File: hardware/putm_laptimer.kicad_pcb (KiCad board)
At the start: 4 copper layers, 76 x 75 mm, 48 parts, among them J1 Conn_01x22, J10 Conn_01x07, J11 Conn_01x09, J12 Conn_01x01, J13 Conn_01x01, J14 Conn_01x01, J15 Conn_01x01, J2 Conn_01x22, J3 Conn_01x22, J4 Conn_01x22, J5 M80-5001805, J6 Conn_02x05_Odd_Even, J7 734-163, J8 734-162, J9 Conn_01x07

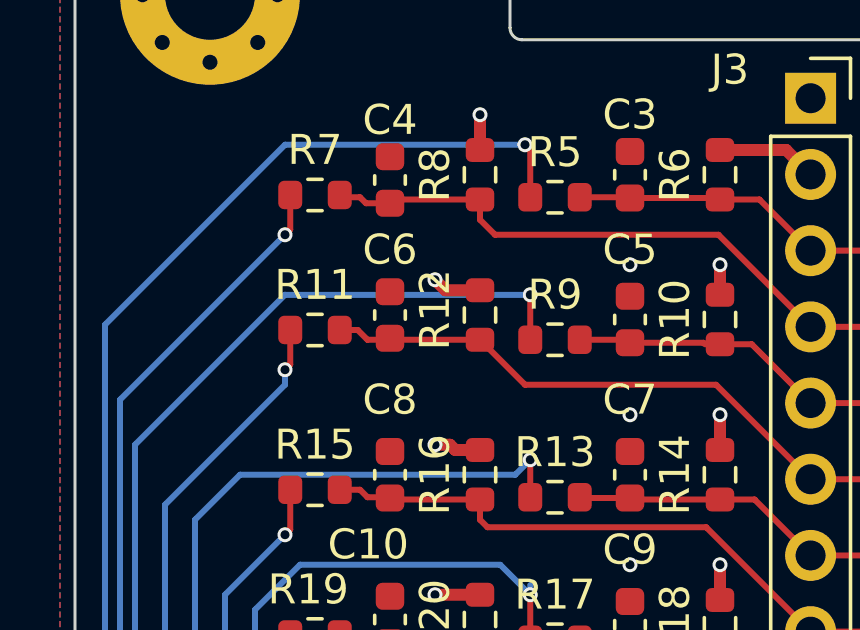
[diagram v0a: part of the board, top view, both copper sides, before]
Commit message: Fixed pcb layout
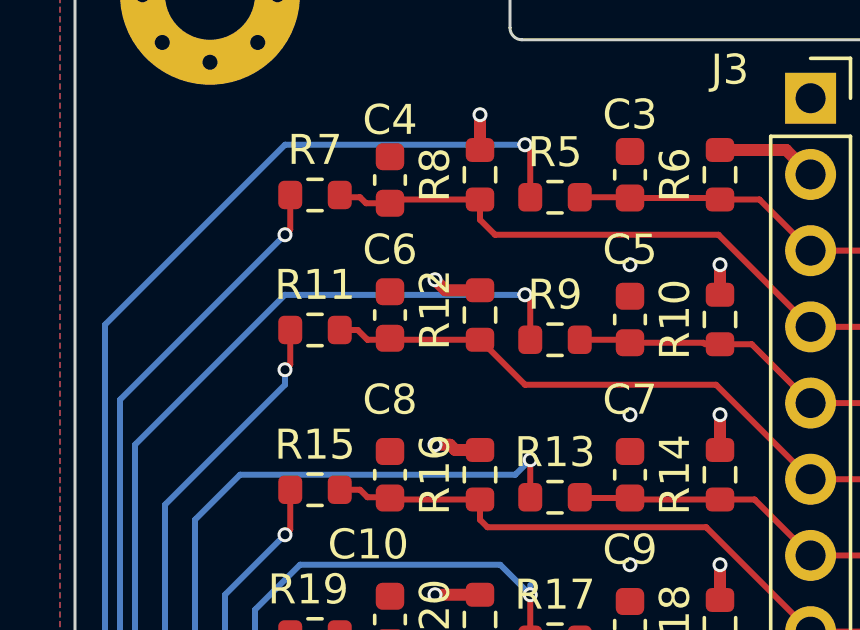
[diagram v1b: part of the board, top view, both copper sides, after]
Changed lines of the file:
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@@
 	)
 	(segment
-		(start 131.175 55.5)
+		(start 131.175 55.675)
 		(end 131.175 57)
 		(width 0.2)
@@
 		(net 32)
 	)
+	(segment
+		(start 131 55.5)
+		(end 131.175 55.675)
+		(width 0.2)
+		(layer "F.Cu")
+		(net 32)
+	)
 	(via
-		(at 131.175 55.5)
+		(at 131 55.5)
 		(size 0.5)
 		(drill 0.3)
 		(layers "F.Cu" "B.Cu")
-		(net 32)
-	)
-	(segment
-		(start 123.005 55.505)
-		(end 123 55.5)
-		(width 0.2)
-		(layer "B.Cu")
-		(net 32)
-	)
-	(segment
-		(start 123 55.5)
-		(end 118 60.5)
-		(width 0.2)
-		(layer "B.Cu")
-		(net 32)
-	)
-	(segment
-		(start 131.17 55.505)
-		(end 123.005 55.505)
-		(width 0.2)
-		(layer "B.Cu")
-		(net 32)
-	)
-	(segment
-		(start 123.5 84)
-		(end 121 86.5)
-		(width 0.2)
-		(layer "B.Cu")
 		(net 32)
 	)
@@
 	)
 	(segment
-		(start 131.175 55.5)
-		(end 131.17 55.505)
+		(start 123 55.5)
+		(end 118 60.5)
 		(width 0.2)
 		(layer "B.Cu")
@@
 		(width 0.2)
 		(layer "B.Cu")
+		(net 32)
+	)
+	(segment
+		(start 130.995 55.505)
+		(end 123.005 55.505)
+		(width 0.2)
+		(layer "B.Cu")
+		(net 32)
+	)
+	(segment
+		(start 123.005 55.505)
+		(end 123 55.5)
+		(width 0.2)
+		(layer "B.Cu")
+		(net 32)
+	)
+	(segment
+		(start 131 55.5)
+		(end 130.995 55.505)
+		(width 0.2)
+		(layer "B.Cu")
+		(net 32)
+	)
+	(segment
+		(start 123.5 84)
+		(end 121 86.5)
+		(width 0.2)
+		(layer "B.Cu")
